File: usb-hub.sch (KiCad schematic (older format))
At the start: 16 parts, among them J1 USB_C_Receptacle_16pin, J5 USB_A socket SMT, U1 fe1-4port-hub, U2 LD1117S12TR_SOT223, Y1 12mhz 20pf

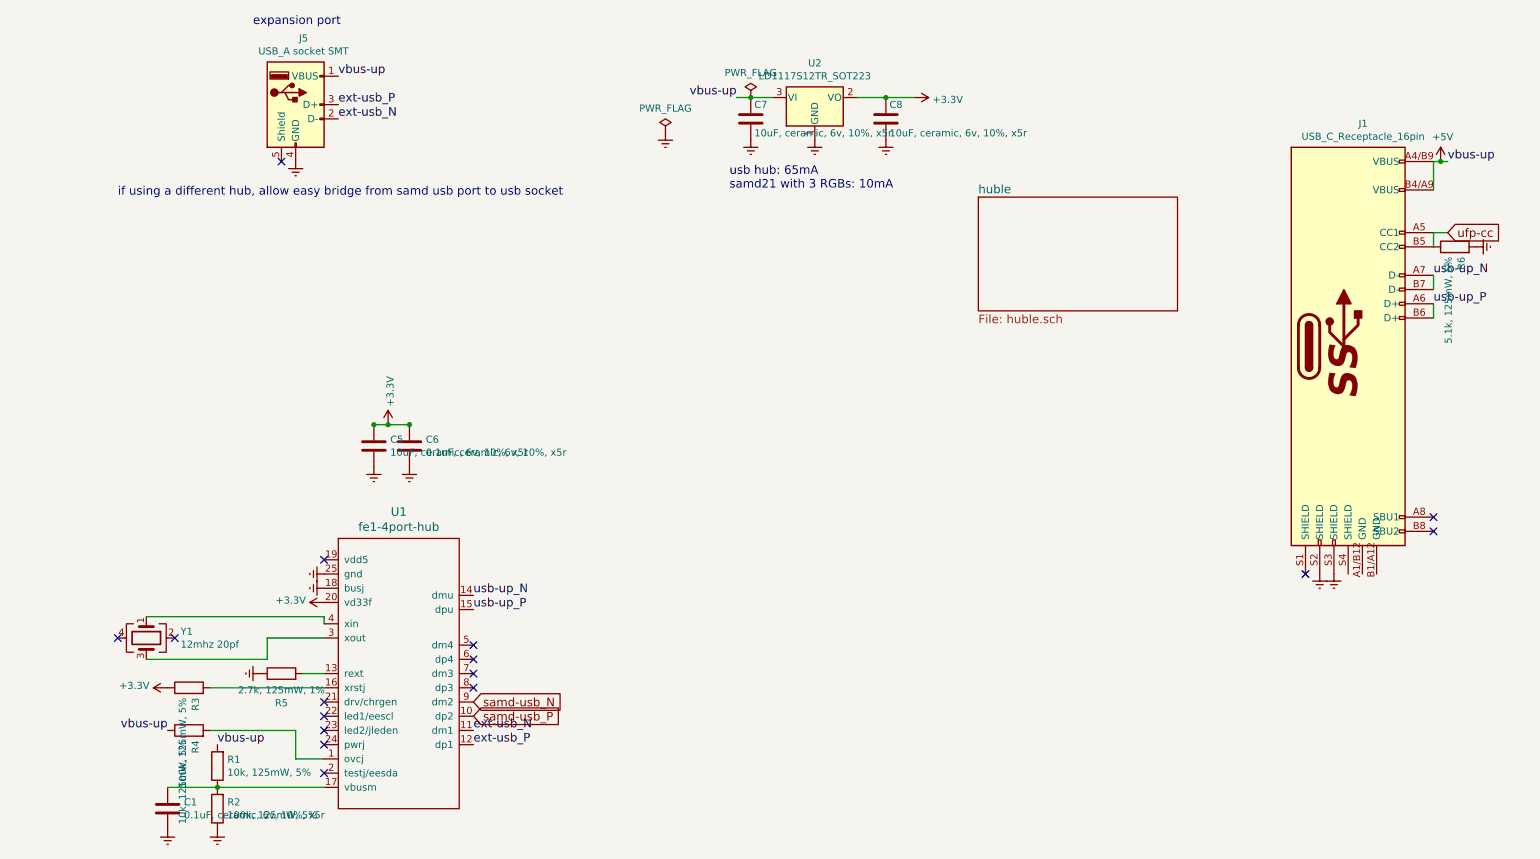
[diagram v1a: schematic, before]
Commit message: differential routing, test pads
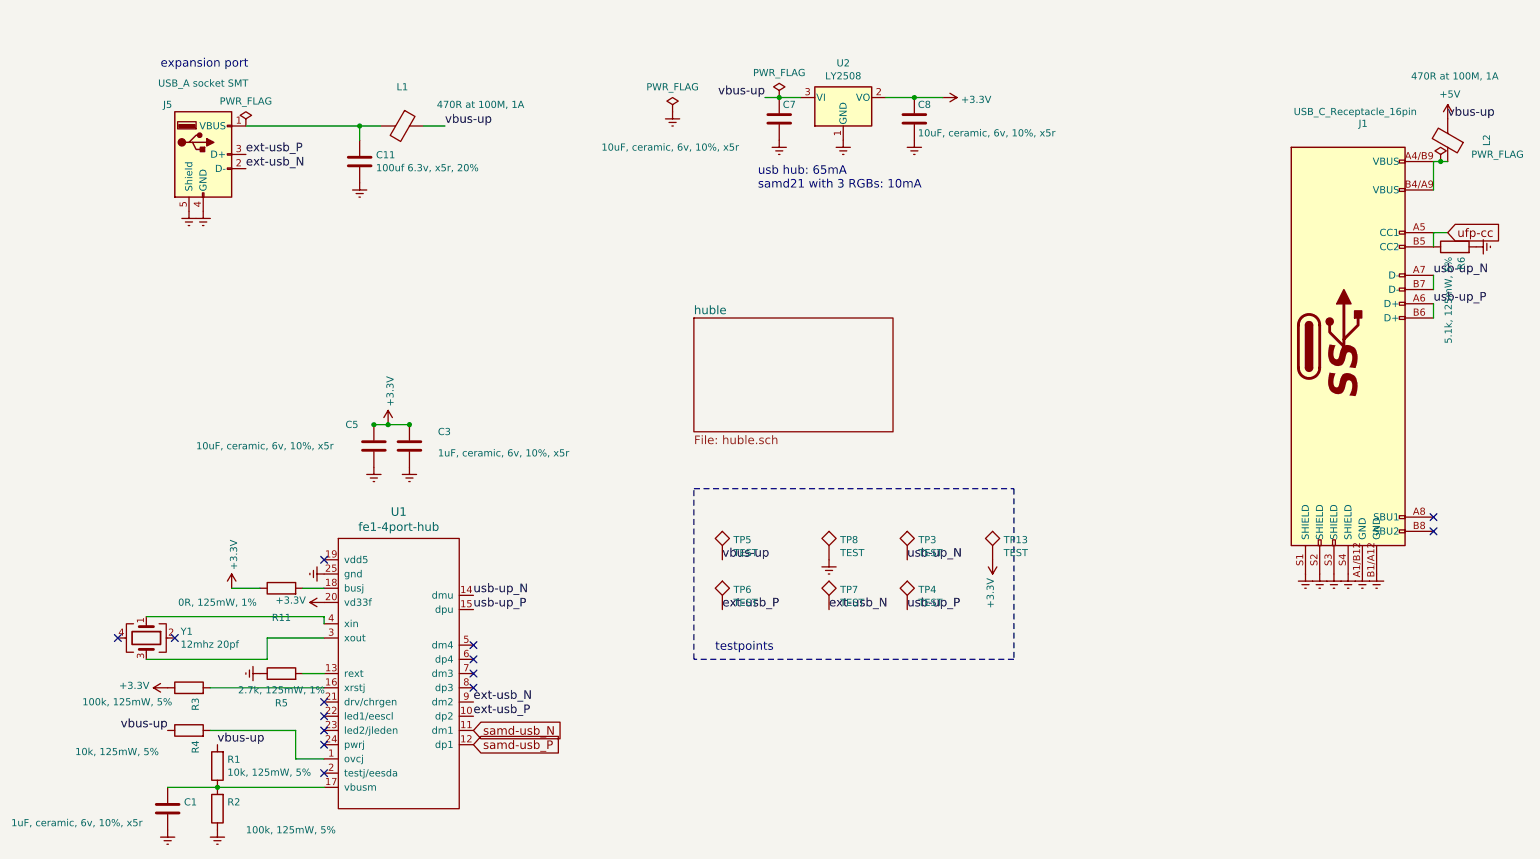
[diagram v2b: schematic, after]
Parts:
- removed C6: 0.1uF, ceramic, 6v, 10%, x5r, Capacitors_SMD:C_0603, symbol C
- added C11: 100uf 6.3v, x5r, 20%, Capacitors_SMD:C_1206, symbol C
- added C3: 1uF, ceramic, 6v, 10%, x5r, Capacitors_SMD:C_0603, symbol C
- added L1, L2: 470R at 100M, 1A, Resistors_SMD:R_0603, symbol Ferrite_Bead
- added R11: 0R, 125mW, 1%, Resistors_SMD:R_0603, symbol R
- added TP13, TP3, TP4, TP5, TP6, TP7, TP8: TEST, fp:testpoint, symbol TEST
- C1: value 0.1uF, ceramic, 6v, 10%, x5r -> 1uF, ceramic, 6v, 10%, x5r; MOQ Value -> (none); farnell # 2522395 -> 1865556; leadtime Value -> (none); supplier PN Value -> (none)
- U2: value LD1117S12TR_SOT223 -> LY2508; footprint TO_SOT_Packages_SMD:SOT-223 -> TO_SOT_Packages_SMD:SOT-23; MOQ (none) -> Value; leadtime (none) -> Value; supplier 低压差线性稳压器 -> Liani; supplier PN HK1117C -> LY2508A33M
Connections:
- net +3V3: now also C3.1, R11.1, TP13.1
- net +5V: now also L1.1, L2.2, TP5.1; no longer J1.A4/B9 (VBUS), J1.B4/A9 (VBUS), J5.1 (VBUS)
- net Earth: now also J1.A1/B12 (GND), J1.B1/A12 (GND), J1.S1 (SHIELD), J1.S4 (SHIELD), J5.5 (Shield), C11.2, C3.2, TP8.1; no longer U1.18 (busj)
- net ext-usb_N: now also U1.9 (dm2), TP7.1; no longer U1.11 (dm1)
- net ext-usb_P: now also U1.10 (dp2), TP6.1; no longer U1.12 (dp1)
- net samd-usb_N: now also U1.11 (dm1); no longer U1.9 (dm2)
- net samd-usb_P: now also U1.12 (dp1); no longer U1.10 (dp2)
- net usb-up_N: now also TP3.1
- net usb-up_P: now also TP4.1
- new net: C11.1, J5.1 (VBUS), L1.2
- new net: J1.A4/B9 (VBUS), J1.B4/A9 (VBUS), L2.1
- new net: R11.2, U1.18 (busj)
- no-connect marks 16 -> 14
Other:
- note added: "testpoints"
- note removed: "if using a different hub, allow easy bridge from samd usb port to usb socket\n"
- moved on the sheet: C7, C8, J5, U2
